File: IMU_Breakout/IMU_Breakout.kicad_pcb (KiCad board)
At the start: 2 copper layers, 10 x 16.8 mm, 4 parts, among them J1 IMU_Connector, U1 LSM6DSL

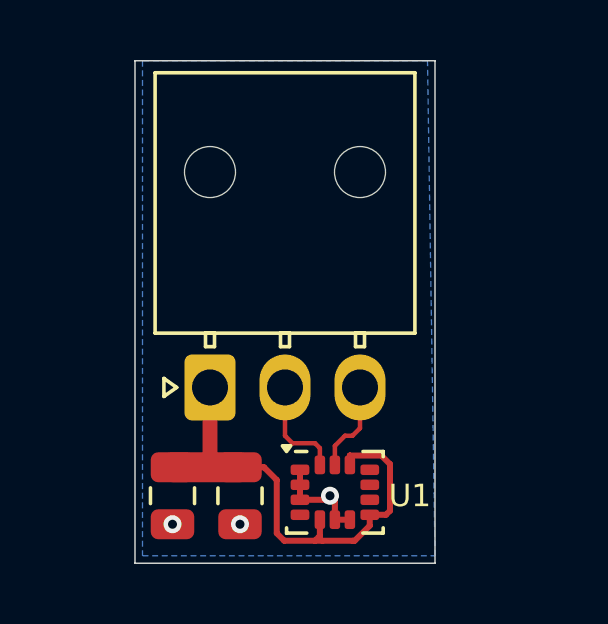
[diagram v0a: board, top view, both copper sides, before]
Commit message: Switched connectors
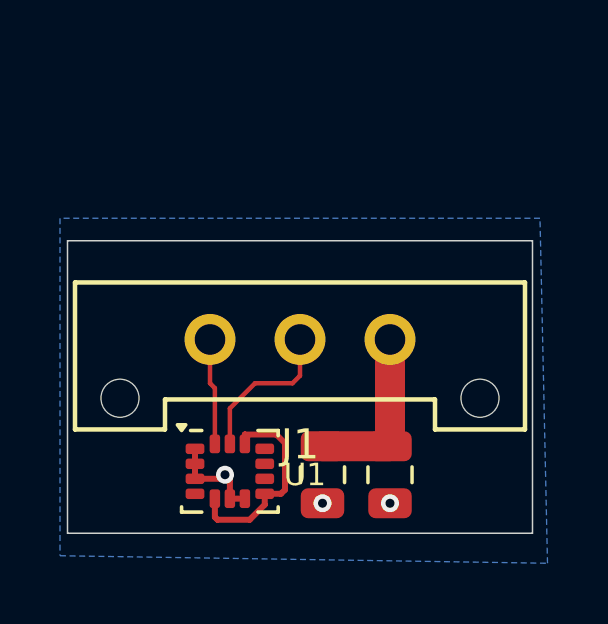
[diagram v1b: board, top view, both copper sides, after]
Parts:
- J1: footprint Connector_Molex:Molex_Nano-Fit_105313-xx03_1x03_P2.50mm_Horizontal -> UTSVT_Connectors:Molex_MicroFit3.0_1x3xP3.00mm_PolarizingPeg_Vertical
- moved J1 6.21 mm to (150.8, 89.3), turned to 180 degrees
- moved C1 5.05 mm to (148.5, 93.8)
- moved C2 5.05 mm to (150.8, 93.8)
- moved U1 3.57 mm to (145.4, 93.7)
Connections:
- J1 pad 2: /IMU_I2C_SDA -> /IMU_I2C_SCL
- J1 pad 3: /IMU_I2C_SCL -> /IMU_I2C_SDA
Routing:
- net /LDO_1.8V: track 17.9 -> 12.5 mm
- net /IMU_I2C_SCL: track 2.97 -> 5.18 mm
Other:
- board size 10 x 16.8 mm -> 15.5 x 9.8 mm
